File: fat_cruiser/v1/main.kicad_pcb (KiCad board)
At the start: 2 copper layers, 222.2 x 100.1 mm, 92 parts

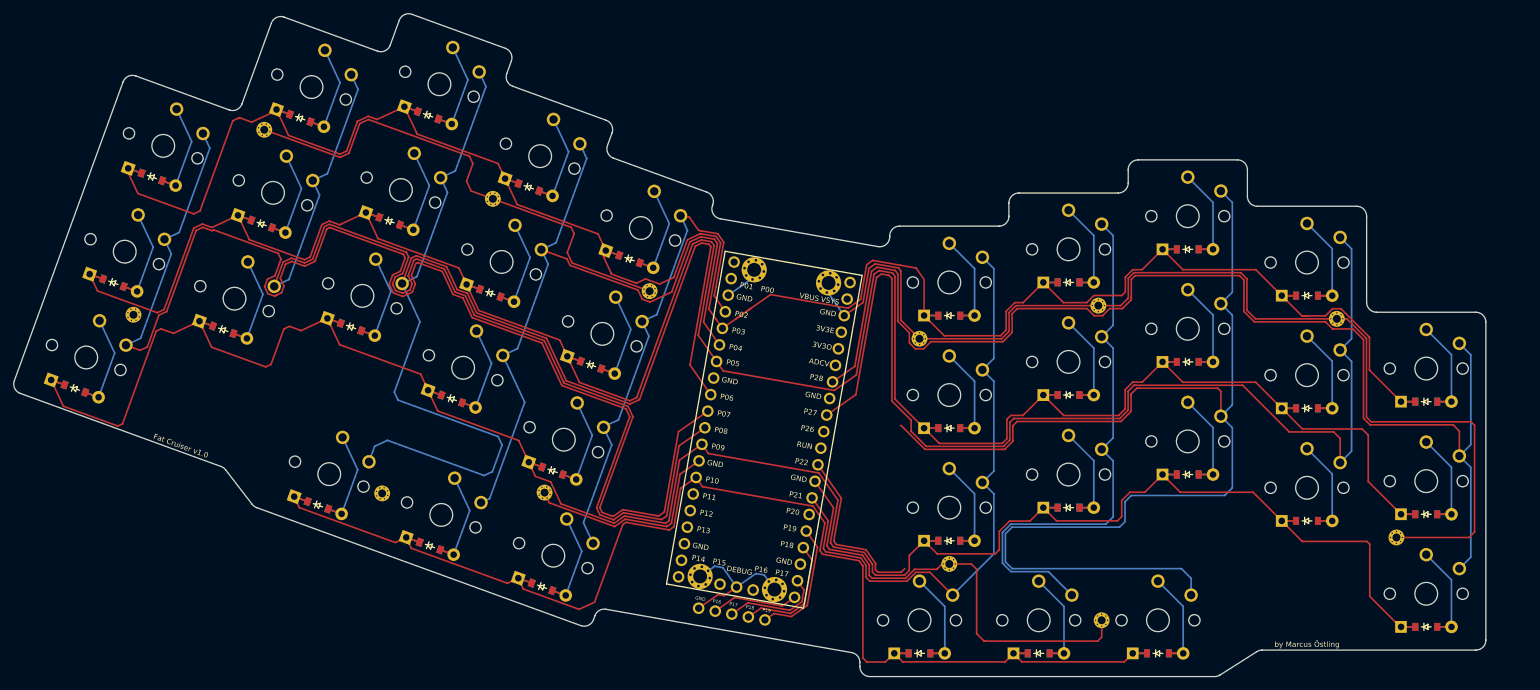
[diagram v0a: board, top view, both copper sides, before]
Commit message: Work on pcb
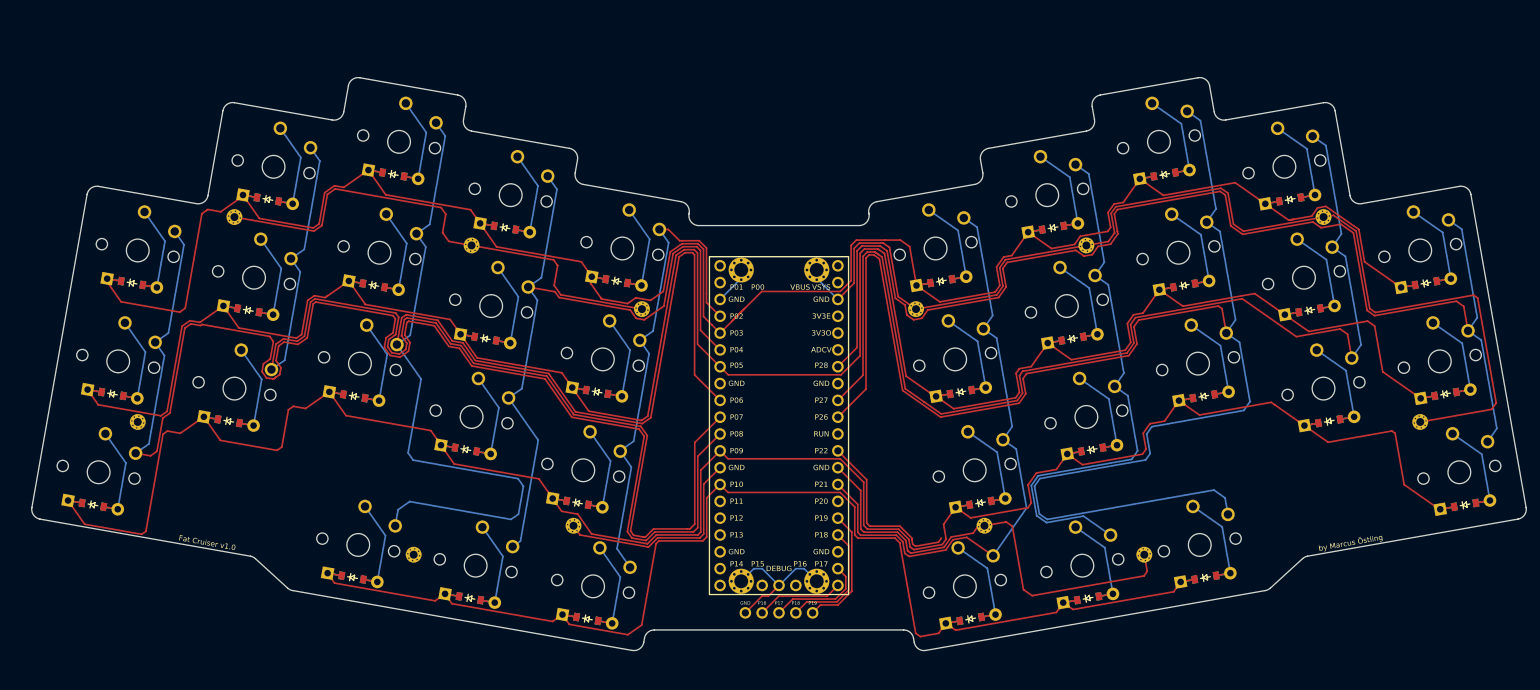
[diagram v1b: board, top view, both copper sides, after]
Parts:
- moved D19 19.3 mm to (261.7, 95.1), turned to 10 degrees
- moved S19 19.0 mm to (260.8, 90.1), turned to 10 degrees
- moved D20 18.4 mm to (258.7, 78.3), turned to 10 degrees
- moved S20 18.2 mm to (257.9, 73.4), turned to 10 degrees
- moved D21 17.9 mm to (255.8, 61.6), turned to 10 degrees
- moved S21 17.8 mm to (254.9, 56.7), turned to 10 degrees
- moved _4 17.8 mm to (254.9, 82.5), turned to 10 degrees
- moved D1 17.8 mm to (54.5, 95.1), turned to -10 degrees
- moved S1 17.4 mm to (55.4, 90.1), turned to -10 degrees
- moved D2 16.8 mm to (57.5, 78.3), turned to -10 degrees
- moved ? 16.7 mm to (244.4, 100.8), turned to 10 degrees
- moved S2 16.6 mm to (58.4, 73.4), turned to -10 degrees
- moved D3 16.3 mm to (60.4, 61.6), turned to -10 degrees
- moved S3 16.3 mm to (61.3, 56.7), turned to -10 degrees
- moved _3 16.2 mm to (61.3, 82.5), turned to -10 degrees
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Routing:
- net P26: track 183.6 -> 233.8 mm
- net P27: track 168.0 -> 168.8 mm
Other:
- board size 222.2 x 100.1 mm -> 225.6 x 86.5 mm
